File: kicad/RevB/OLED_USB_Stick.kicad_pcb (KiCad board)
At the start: 2 copper layers, 62.5 x 14.7 mm, 31 parts, among them J1 USB_A, J3 Conn_01x04, SW1 SW_SPDT, SW2 SW_SPST, U1 FT232RL, U2 SE8233X2, U3 STM32F051K4Tx

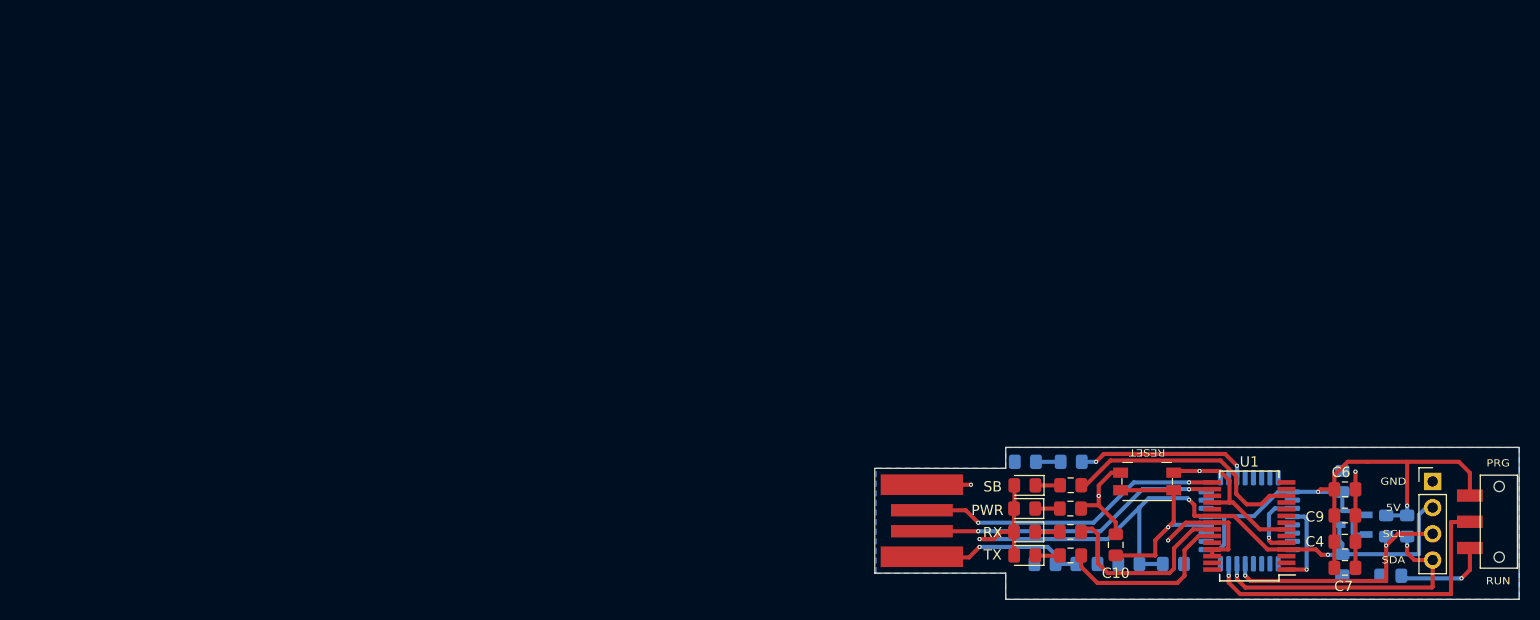
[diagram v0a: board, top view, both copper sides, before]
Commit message: update readme
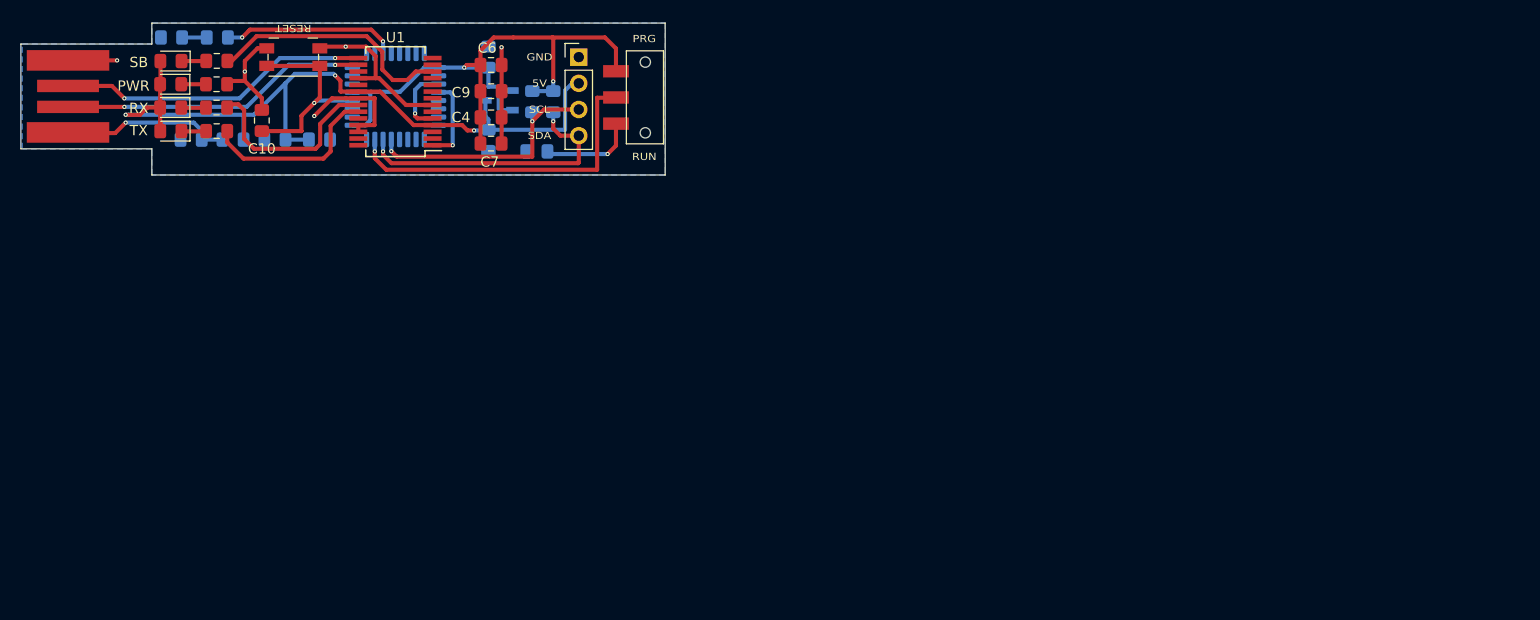
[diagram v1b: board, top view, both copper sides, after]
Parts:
- moved C10 92.5 mm to (65.5, 39.9)
- moved C4 92.5 mm to (87.8, 39.6)
- moved D1 92.5 mm to (56.7, 41.0)
- moved D2 92.5 mm to (56.7, 38.7)
- moved D3 92.5 mm to (56.7, 34.2)
- moved D5 92.5 mm to (61.2, 31.9)
- moved R1 92.5 mm to (61.2, 41.0)
- moved R2 92.5 mm to (61.1, 38.7)
- moved R6 92.5 mm to (91.8, 38.1)
- moved R7 92.5 mm to (93.8, 38.1)
- moved R8 92.5 mm to (56.8, 31.9)
- moved C1 92.5 mm to (58.7, 41.8)
- moved C2 92.5 mm to (66.8, 41.8)
- moved C3 92.5 mm to (71.1, 41.8)
- moved C5 92.5 mm to (87.5, 41.8)
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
